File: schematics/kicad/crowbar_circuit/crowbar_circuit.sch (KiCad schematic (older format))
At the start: 2 parts

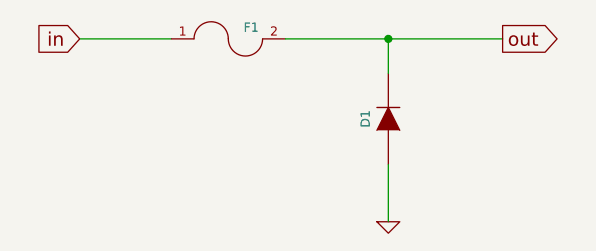
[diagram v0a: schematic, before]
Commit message: schéma jolis pour les screenshot, et screenshots
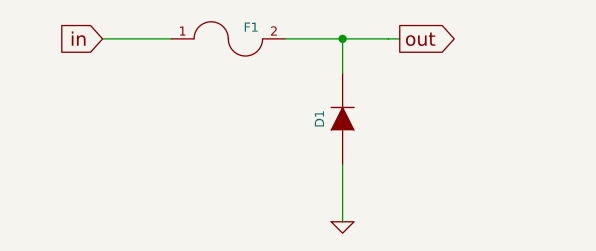
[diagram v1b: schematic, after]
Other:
- moved on the sheet: D1
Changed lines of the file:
@@
 Sheet 1 1
 Title ""
-Date "9 sep 2015"
+Date "12 sep 2015"
 Rev ""
 Comp ""
@@
 L DIODE D1
 U 1 1 55F08AEA
-P 3750 3050
-F 0 "D1" H 3750 3150 40  0000 C CNN
-F 1 " " H 3750 2950 40  0000 C CNN
-F 2 "~" H 3750 3050 60  0000 C CNN
-F 3 "~" H 3750 3050 60  0000 C CNN
-	1    3750 3050
+P 3550 3050
+F 0 "D1" H 3550 3150 40  0000 C CNN
+F 1 " " H 3550 2950 40  0000 C CNN
+F 2 "~" H 3550 3050 60  0000 C CNN
+F 3 "~" H 3550 3050 60  0000 C CNN
+	1    3550 3050
 	0    -1   -1   0
 $EndComp
@@
 L GND #PWR?
 U 1 1 55F08AF9
-P 3750 3500
-F 0 "#PWR?" H 3750 3500 30  0001 C CNN
-F 1 "GND" H 3750 3430 30  0001 C CNN
-F 2 "" H 3750 3500 60  0000 C CNN
-F 3 "" H 3750 3500 60  0000 C CNN
-	1    3750 3500
+P 3550 3500
+F 0 "#PWR?" H 3550 3500 30  0001 C CNN
+F 1 "GND" H 3550 3430 30  0001 C CNN
+F 2 "" H 3550 3500 60  0000 C CNN
+F 3 "" H 3550 3500 60  0000 C CNN
+	1    3550 3500
 	1    0    0    -1
 $EndComp
-Text GLabel 2400 2700 0    60   Input ~ 0
+Text GLabel 2500 2700 0    60   Input ~ 0
 in
-Text GLabel 4250 2700 2    60   Output ~ 0
+Text GLabel 3800 2700 2    60   Output ~ 0
 out
 Wire Wire Line
-	2400 2700 2800 2700
+	2500 2700 2800 2700
 Wire Wire Line
-	3300 2700 4250 2700
+	3300 2700 3550 2700
 Wire Wire Line
-	3750 2850 3750 2700
-Connection ~ 3750 2700
+	3550 2700 3550 2700
 Wire Wire Line
-	3750 3250 3750 3500
+	3550 2700 3750 2700
+Wire Wire Line
+	3750 2700 3800 2700
+Wire Wire Line
+	3550 2850 3550 2700
+Wire Wire Line
+	3550 3250 3550 3500
+Connection ~ 3550 2700
 $EndSCHEMATC
